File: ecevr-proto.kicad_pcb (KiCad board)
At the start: 4 copper layers, 100 x 92 mm, 218 parts, among them J1 Micro_SD_Card_Det, J1101 USB_microB, J1102 USB_C_Receptacle_USB2.0, J19 SFP, J2 Pwr_fallback, J20 SFP_CAGE, J2001 BNC, J2051 BNC, J2201 BEL_0845_2G1T_H5, J4 JTAG, J5 0821-1X1T-43-F, SW1 SW_Push, SW2101 SW_DIP_x08, U1 TXS0108EPW, U1101 USB3740B-AI9, U1102 UTC2000, U1103 FT231XS, U1104 74LVC1G00, U1105 SC185, U2001 74LVC2T45DC, U2051 74LVC2T45DC, U2101 74LVC1G06, U2102 74LVC1G06, U2103 PCA9306, U2104 24AA0x, U2201 74LVC1G06, U2202 74LVC1G06, U2301 lan9254, U6 PCA9546AD, U8 74AC125, U9 TPS2051B, X2301 FNETHE025

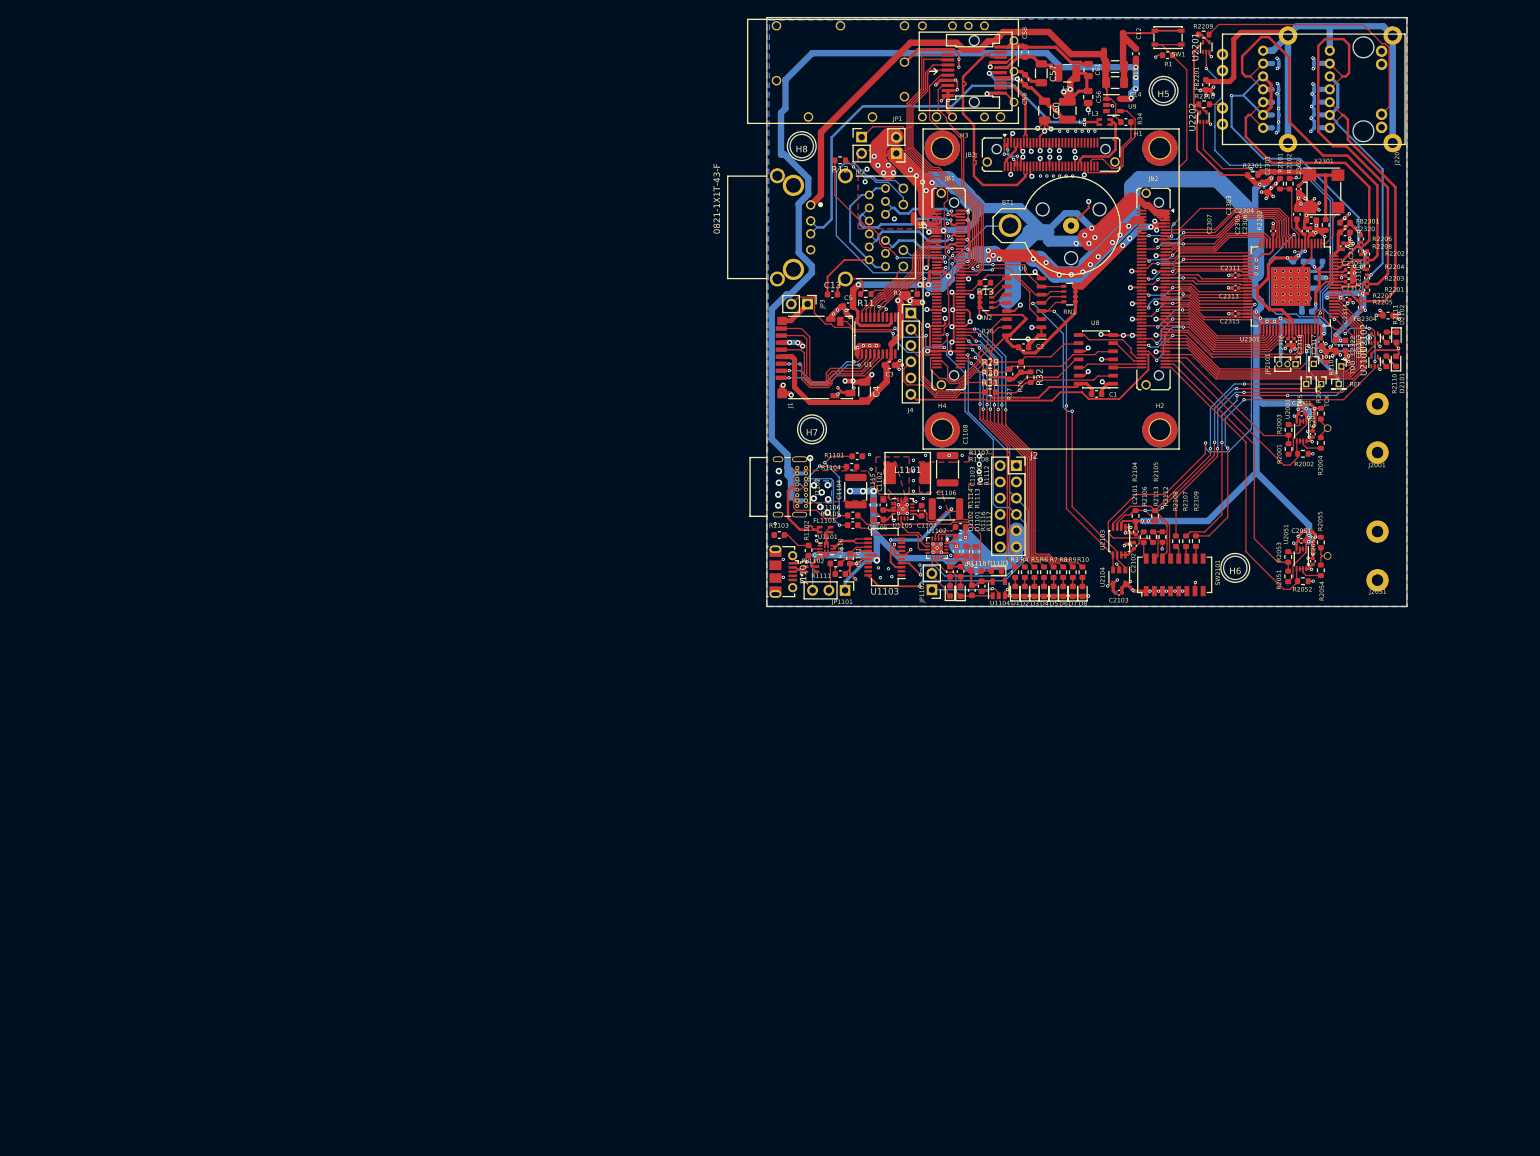
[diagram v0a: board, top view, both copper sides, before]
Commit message: WIP: (save)
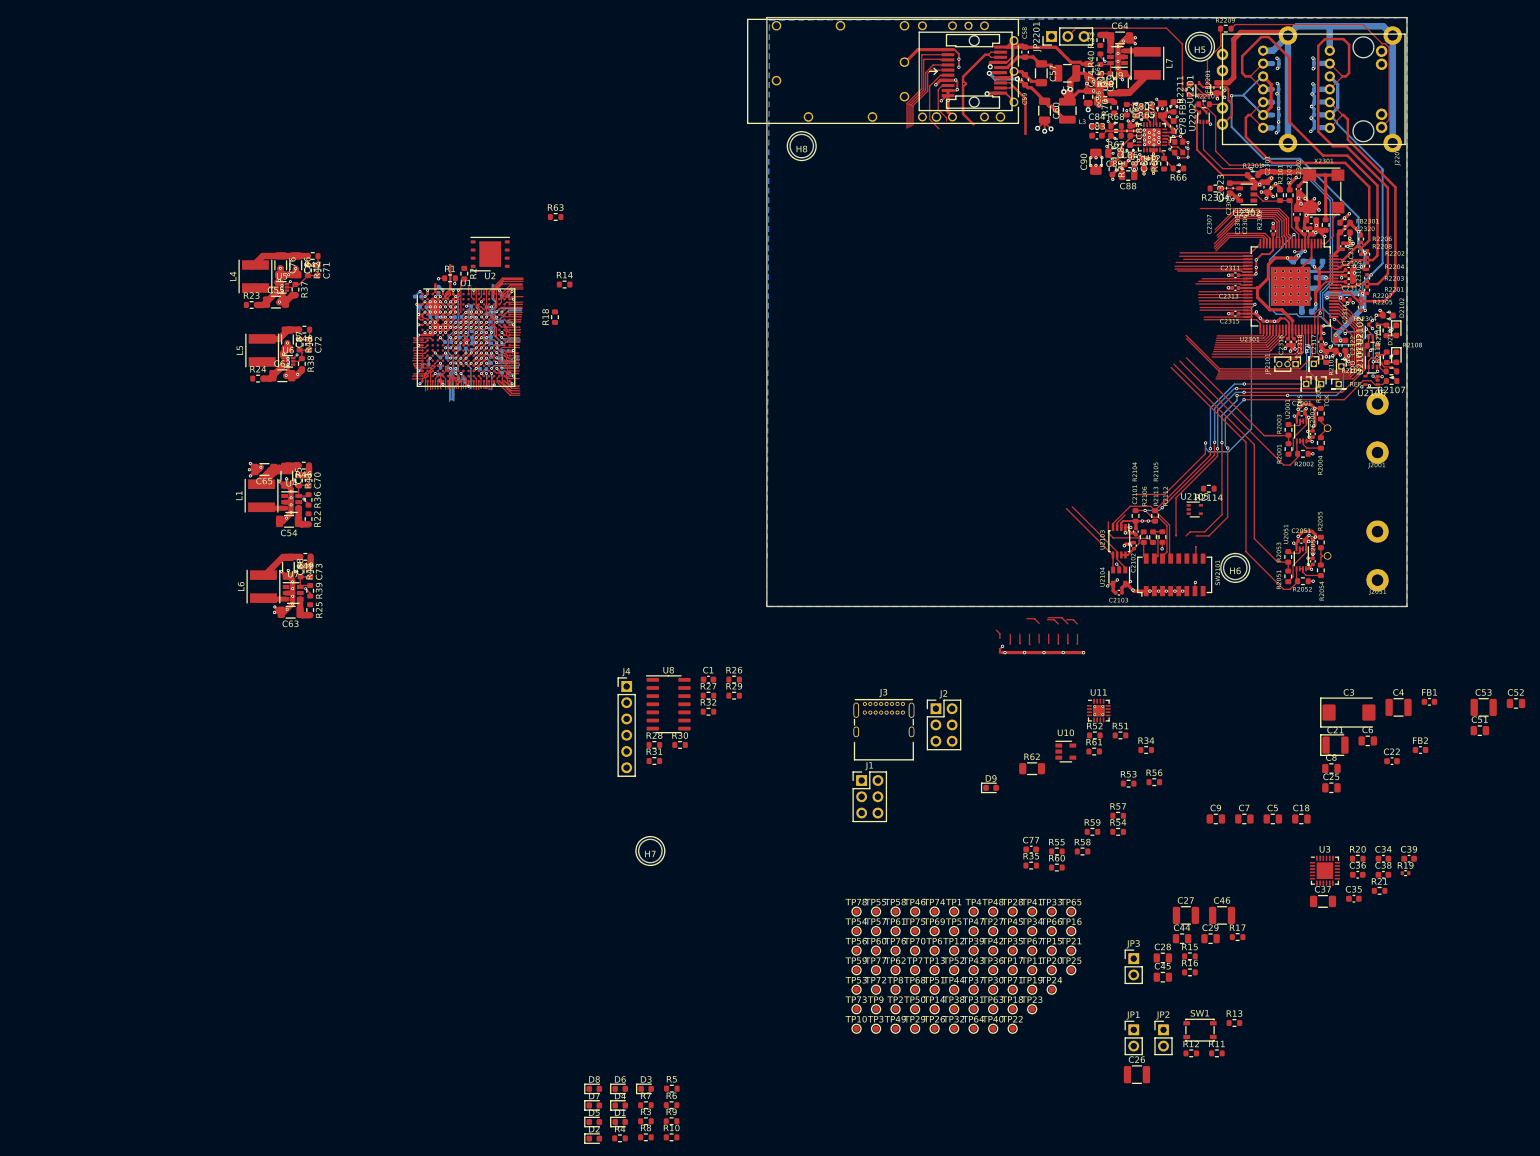
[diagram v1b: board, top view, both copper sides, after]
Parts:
- removed BT1: CR1220, Battery:BatteryHolder_Keystone_500
- removed C1101, C1102, C1103, C1105, C1107: 100nF_603, Capacitor_SMD:C_0603_1608Metric
- removed C1104, C1106, C1108: 22uF_lo_ESR, Capacitor_SMD:C_1812_4532Metric
- removed D1101, D1102, D1103: LED, LED_SMD:LED_0603_1608Metric
- removed FL1101, FL1102, FL3: EMI_Filter_LL_14, proj_footprints:WE_CNSW
- removed H1, H2, H3, H4: MountingHole_Pad, MountingHole:MountingHole_3.2mm_M3_ISO14580_Pad_TopBottom
- removed J1101: USB_microB, Connector_USB:USB_Micro-B_Molex-105017-0001
- removed J1102: USB_C_Receptacle_USB2.0, proj_footprints:USB_C_Receptacle_GCT_USB4085_smaller_holes
- removed J5: 0821-1X1T-43-F, proj_footprints:BEL_0821-1X1T-43-F
- removed JB1: LSHM-150-04_JB1, Connector_Samtec:Samtec_LSHM-150-xx.x-x-DV-S_2x50-1SH_P0.50mm_Vertical
- removed JB2: LSHM-150-04_JB2, Connector_Samtec:Samtec_LSHM-150-xx.x-x-DV-S_2x50-1SH_P0.50mm_Vertical
- removed JB3: LSHM-130-04_JB3, Connector_Samtec:Samtec_LSHM-130-xx.x-x-DV-S_2x30-1SH_P0.50mm_Vertical
- removed JP1101: Jumper_3_Bridged12, Connector_PinHeader_2.54mm:PinHeader_1x03_P2.54mm_Vertical
- removed JP1102: Jumper_NO_Small, Connector_PinHeader_2.54mm:PinHeader_1x02_P2.54mm_Vertical
- removed L1101: 1uH, proj_footprints:L_TDK_SPM6530
- removed R1101, R1104, R1109, R1110: 5k1, Resistor_SMD:R_0603_1608Metric
- removed R1102, R1103, R1116, R1117: 100k, Resistor_SMD:R_0603_1608Metric
- removed R1105, R1106, R1107, R1108, R1111: 10k, Resistor_SMD:R_0603_1608Metric
- removed R1112: 35k7, Resistor_SMD:R_0603_1608Metric
- removed R1113, R1114, R1118: 1k, Resistor_SMD:R_0603_1608Metric
- removed R1115: 1, Resistor_SMD:R_0603_1608Metric
- removed RN1, RN2: 4x4k7, Resistor_SMD:R_Array_Convex_4x0603
- removed U1101: USB3740B-AI9, Package_DFN_QFN:UQFN-10_1.6x2.1mm_P0.5mm
- removed U1102: UTC2000, proj_footprints:QFN-16-1EP_3x3mm_P0.5mm_EP1.8x1.8mm
- removed U1103: FT231XS, Package_SO:SSOP-20_3.9x8.7mm_P0.635mm
- removed U1104: 74LVC1G00, Package_TO_SOT_SMD:SOT-23-5
- removed U1105: SC185, proj_footprints:QFN-16-1EP_3x3mm_P0.5mm_EP1.8x1.8mm
- added C10: 470n, Capacitor_SMD:C_0402_1005Metric, B.Cu at (56.9, 78.0)
- added C11: 100n, Capacitor_SMD:C_0402_1005Metric, B.Cu at (48.7, 72.5)
- added C16: 470n, Capacitor_SMD:C_0402_1005Metric, B.Cu at (56.9, 83.5)
- added C17: 470n, Capacitor_SMD:C_0402_1005Metric, B.Cu at (52.5, 81.7)
- added C18: 4u7, Capacitor_SMD:C_0805_2012Metric, F.Cu at (183.5, 155.2)
- added C19: 470n, Capacitor_SMD:C_0402_1005Metric, B.Cu at (53.9, 79.5)
- added C20: 470n, Capacitor_SMD:C_0402_1005Metric, B.Cu at (53.9, 81.4)
- added C21: 100u, proj_footprints:C_pol_1210_3225Metric, F.Cu at (188.8, 143.7)
- added C22: 470n, Capacitor_SMD:C_0603_1608Metric, F.Cu at (197.7, 146.2)
- added C23: 100n, Capacitor_SMD:C_0402_1005Metric, B.Cu at (45.5, 73.6)
- added C2323: 100n, Capacitor_SMD:C_0603_1608Metric, F.Cu at (172.3, 56.6)
- added C24: 100n, Capacitor_SMD:C_0402_1005Metric, B.Cu at (46.3, 75.2)
- added C25: 4u7, Capacitor_SMD:C_0805_2012Metric, F.Cu at (188.2, 150.3)
- added C26: 47u, Capacitor_SMD:C_1210_3225Metric, F.Cu at (157.8, 195.1)
- added C27: 47u, Capacitor_SMD:C_1210_3225Metric, F.Cu at (165.5, 170.3)
- added C28: 4u7, Capacitor_SMD:C_0805_2012Metric, F.Cu at (161.9, 176.9)
- added C29: 4u7, Capacitor_SMD:C_0805_2012Metric, F.Cu at (169.3, 173.9)
- added C30: 470n, Capacitor_SMD:C_0402_1005Metric, B.Cu at (59.1, 82.1)
- added C31: 470n, Capacitor_SMD:C_0402_1005Metric, B.Cu at (59.1, 85.5)
- added C32: 470n, Capacitor_SMD:C_0402_1005Metric, B.Cu at (52.3, 86.4)
- added C33: 470n, Capacitor_SMD:C_0402_1005Metric, B.Cu at (55.7, 84.9)
- added C34: 47p, Capacitor_SMD:C_0603_1608Metric, F.Cu at (196.3, 161.4)
- added C35: 47p, Capacitor_SMD:C_0603_1608Metric, F.Cu at (191.7, 167.7)
- added C36: 100n, Capacitor_SMD:C_0603_1608Metric, F.Cu at (192.3, 163.9)
- added C37: 10u, Capacitor_SMD:C_1206_3216Metric, F.Cu at (186.9, 168.1)
- added C38: 100n, Capacitor_SMD:C_0603_1608Metric, F.Cu at (196.3, 163.9)
- added C39: 100n, Capacitor_SMD:C_0603_1608Metric, F.Cu at (200.3, 161.4)
- added C40: 470n, Capacitor_SMD:C_0402_1005Metric, B.Cu at (56.2, 75.7)
- added C41: 470n, Capacitor_SMD:C_0402_1005Metric, B.Cu at (59.1, 77.5)
- added C42: 470n, Capacitor_SMD:C_0402_1005Metric, B.Cu at (59.1, 73.5)
- added C43: 470n, Capacitor_SMD:C_0402_1005Metric, B.Cu at (54.3, 75.1)
- added C44: 4u7, Capacitor_SMD:C_0805_2012Metric, F.Cu at (164.9, 173.9)
- added C45: 4u7, Capacitor_SMD:C_0805_2012Metric, F.Cu at (161.9, 179.9)
- added C46: 47u, Capacitor_SMD:C_1210_3225Metric, F.Cu at (171.1, 170.3)
- added C47: 470n, Capacitor_SMD:C_0402_1005Metric, B.Cu at (49.5, 83.1)
- added C48: 470n, Capacitor_SMD:C_0402_1005Metric, B.Cu at (49.5, 84.7)
- added C49: 470n, Capacitor_SMD:C_0402_1005Metric, B.Cu at (46.7, 84.2)
- added C50: 470n, Capacitor_SMD:C_0402_1005Metric, B.Cu at (48.9, 86.2)
- added C51: 4u7, Capacitor_SMD:C_0805_2012Metric, F.Cu at (211.4, 141.4)
- added C52: 4u7, Capacitor_SMD:C_0805_2012Metric, F.Cu at (217.0, 137.2)
- added C53: 47u, Capacitor_SMD:C_1210_3225Metric, F.Cu at (212.0, 137.8)
- added C54: 10u, Capacitor_SMD:C_1206_3216Metric, F.Cu at (25.4, 108.7)
- added C55: 10u, Capacitor_SMD:C_1206_3216Metric, F.Cu at (23.3, 74.5)
- added C6: 4u7, Capacitor_SMD:C_0805_2012Metric, F.Cu at (193.9, 143.0)
- added C62: 10u, Capacitor_SMD:C_1206_3216Metric, F.Cu at (24.3, 86.0)
- added C63: 10u, Capacitor_SMD:C_1206_3216Metric, F.Cu at (25.6, 122.9)
- added C64: 10u, Capacitor_SMD:C_1206_3216Metric, F.Cu at (155.2, 33.2)
- added C65: 22u, Capacitor_SMD:C_1206_3216Metric, F.Cu at (21.5, 100.6)
- added C66: 22u, Capacitor_SMD:C_1206_3216Metric, F.Cu at (26.4, 68.7)
- added C67: 22u, Capacitor_SMD:C_1206_3216Metric, F.Cu at (25.1, 80.3)
- added C68: 10u, Capacitor_SMD:C_1206_3216Metric, F.Cu at (25.2, 115.8)
- added C69: 10u, Capacitor_SMD:C_1206_3216Metric, F.Cu at (155.6, 40.2)
- added C7: 4u7, Capacitor_SMD:C_0805_2012Metric, F.Cu at (174.6, 155.2)
- added C70: 86p, Capacitor_SMD:C_0603_1608Metric, F.Cu at (28.4, 102.3)
- added C71: 86p, Capacitor_SMD:C_0603_1608Metric, F.Cu at (29.8, 69.5)
- added C72: 56p, Capacitor_SMD:C_0603_1608Metric, F.Cu at (28.5, 81.1)
- added C73: 56p, Capacitor_SMD:C_0603_1608Metric, F.Cu at (28.6, 116.6)
- added C74: 130p, Capacitor_SMD:C_0603_1608Metric, F.Cu at (152.2, 39.5)
- added C75: 22u, Capacitor_SMD:C_1206_3216Metric, F.Cu at (25.0, 101.6)
- added C76: 22u, Capacitor_SMD:C_1206_3216Metric, F.Cu at (24.1, 68.7)
- added C77: 100n, Capacitor_SMD:C_0603_1608Metric, F.Cu at (141.3, 160.0)
- added C78: 100n, Capacitor_SMD:C_0603_1608Metric, F.Cu at (163.6, 47.0)
- added C79: 1u, Capacitor_SMD:C_0805_2012Metric, F.Cu at (161.8, 44.4)
- added C8: 4u7, Capacitor_SMD:C_0805_2012Metric, F.Cu at (188.2, 147.3)
- added C80: 100n, Capacitor_SMD:C_0603_1608Metric, F.Cu at (158.4, 45.4)
- added C81: 100n, Capacitor_SMD:C_0603_1608Metric, F.Cu at (156.8, 50.7)
- added C82: 100n, Capacitor_SMD:C_0603_1608Metric, F.Cu at (160.4, 52.8)
- added C83: C_Small, Capacitor_SMD:C_0603_1608Metric, F.Cu at (151.6, 48.5)
- added C84: C_Small, Capacitor_SMD:C_0603_1608Metric, F.Cu at (151.6, 47.0)
- added C85: 100n, Capacitor_SMD:C_0603_1608Metric, F.Cu at (158.9, 52.8)
- added C86: 100n, Capacitor_SMD:C_0603_1608Metric, F.Cu at (156.7, 52.9)
- added C87: 100n, Capacitor_SMD:C_0603_1608Metric, F.Cu at (156.8, 47.7)
- added C88: 1u, Capacitor_SMD:C_0805_2012Metric, F.Cu at (156.4, 54.7)
- added C89: 1u, Capacitor_SMD:C_0805_2012Metric, F.Cu at (154.3, 51.2)
- added C9: 4u7, Capacitor_SMD:C_0805_2012Metric, F.Cu at (170.1, 155.2)
- added C90: 10u, Capacitor_SMD:C_1206_3216Metric, F.Cu at (151.4, 52.5)
- added D9: LED, LED_SMD:LED_0603_1608Metric, F.Cu at (135.0, 150.3)
- added FB1: FB_250, Inductor_SMD:L_0603_1608Metric, F.Cu at (203.5, 136.9)
- added FB2: FB_250, Inductor_SMD:L_0603_1608Metric, F.Cu at (202.1, 144.4)
- added FB3: Ferrite_Bead, Inductor_SMD:L_0603_1608Metric, F.Cu at (163.6, 44.0)
- added J3: USB_C_Receptacle_USB2.0, proj_footprints:USB_C_Receptacle_GCT_USB4085_smaller_holes, F.Cu at (115.3, 137.2)
- added JP2201: 100FDb, Connector_PinHeader_2.54mm:PinHeader_1x03_P2.54mm_Vertical, F.Cu at (144.5, 33.0)
- added L1: 2u2, Inductor_SMD:L_Taiyo-Yuden_NR-50xx, F.Cu at (21.1, 104.7)
- added L4: 1u, Inductor_SMD:L_Taiyo-Yuden_NR-50xx, F.Cu at (20.1, 70.5)
- added L5: 1u, Inductor_SMD:L_Taiyo-Yuden_NR-50xx, F.Cu at (21.1, 82.0)
- added L6: 2u2, Inductor_SMD:L_Taiyo-Yuden_NR-50xx, F.Cu at (21.4, 118.9)
- added L7: 2u2, Inductor_SMD:L_Taiyo-Yuden_NR-50xx, F.Cu at (159.4, 37.1)
- added R14: 1k, Resistor_SMD:R_0603_1608Metric, F.Cu at (68.4, 71.7)
- added R15: 2k4, Resistor_SMD:R_0603_1608Metric, F.Cu at (166.1, 176.7)
- added R16: 2k4, Resistor_SMD:R_0603_1608Metric, F.Cu at (166.1, 179.2)
- added R17: 2k4, Resistor_SMD:R_0603_1608Metric, F.Cu at (173.5, 173.7)
- added R18: 50, Resistor_SMD:R_0603_1608Metric, F.Cu at (66.9, 76.8)
- added R19: 0, Resistor_SMD:R_0402_1005Metric, F.Cu at (199.8, 163.7)
- added R20: 27, Resistor_SMD:R_0603_1608Metric, F.Cu at (192.3, 161.4)
- added R21: 27, Resistor_SMD:R_0603_1608Metric, F.Cu at (195.7, 166.4)
- added R2114: 100k, Resistor_SMD:R_0603_1608Metric, F.Cu at (169.1, 103.6)
- added R22: 10k, Resistor_SMD:R_0603_1608Metric, F.Cu at (28.4, 108.3)
- added R2211: 100, Resistor_SMD:R_0603_1608Metric, F.Cu at (166.0, 41.2)
- added R23: 10k, Resistor_SMD:R_0603_1608Metric, F.Cu at (19.5, 74.9)
- added R2304: 50, Resistor_SMD:R_0603_1608Metric, F.Cu at (170.1, 56.7)
- added R24: 10k, Resistor_SMD:R_0603_1608Metric, F.Cu at (20.5, 86.4)
- added R25: 10k, Resistor_SMD:R_0603_1608Metric, F.Cu at (28.6, 122.5)
- added R33: 10k, Resistor_SMD:R_0603_1608Metric, F.Cu at (152.1, 33.5)
- added R35: 10k, Resistor_SMD:R_0603_1608Metric, F.Cu at (141.3, 162.5)
- added R36: 24k, Resistor_SMD:R_0603_1608Metric, F.Cu at (28.4, 105.3)
- added R37: 24k, Resistor_SMD:R_0603_1608Metric, F.Cu at (26.4, 72.5)
- added R38: 24k, Resistor_SMD:R_0603_1608Metric, F.Cu at (27.4, 84.1)
- added R39: 12k, Resistor_SMD:R_0603_1608Metric, F.Cu at (28.6, 119.5)
- added R40: 45.9k, Resistor_SMD:R_0603_1608Metric, F.Cu at (152.1, 36.5)
- added R41: 16k, Resistor_SMD:R_0603_1608Metric, F.Cu at (26.9, 102.3)
- added R42: 16k, Resistor_SMD:R_0603_1608Metric, F.Cu at (28.3, 69.5)
- added R43: 24k, Resistor_SMD:R_0603_1608Metric, F.Cu at (27.0, 81.1)
- added R44: 24k, Resistor_SMD:R_0603_1608Metric, F.Cu at (27.1, 116.5)
- added R45: 10.2k, Resistor_SMD:R_0603_1608Metric, F.Cu at (153.7, 39.5)
- added R46: 0, Resistor_SMD:R_0603_1608Metric, F.Cu at (27.6, 100.0)
- added R47: 0, Resistor_SMD:R_0603_1608Metric, F.Cu at (29.1, 67.2)
- added R48: 0, Resistor_SMD:R_0603_1608Metric, F.Cu at (27.8, 78.8)
- added R49: 0, Resistor_SMD:R_0603_1608Metric, F.Cu at (27.9, 114.2)
- added R50: 0, Resistor_SMD:R_0603_1608Metric, F.Cu at (152.9, 41.8)
- added R51: 1k, Resistor_SMD:R_0603_1608Metric, F.Cu at (155.2, 142.2)
- added R52: 100k, Resistor_SMD:R_0603_1608Metric, F.Cu at (151.2, 142.2)
- added R53: 100k, Resistor_SMD:R_0603_1608Metric, F.Cu at (156.5, 149.7)
- added R54: 10k, Resistor_SMD:R_0603_1608Metric, F.Cu at (154.9, 157.2)
- added R55: 10k, Resistor_SMD:R_0603_1608Metric, F.Cu at (145.3, 160.3)
- added R56: 5k1, Resistor_SMD:R_0603_1608Metric, F.Cu at (160.5, 149.4)
- added R57: 5k1, Resistor_SMD:R_0603_1608Metric, F.Cu at (154.9, 154.7)
- added R58: 10k, Resistor_SMD:R_0603_1608Metric, F.Cu at (149.3, 160.3)
- added R59: 10k, Resistor_SMD:R_0603_1608Metric, F.Cu at (150.9, 157.2)
- added R60: 5k1, Resistor_SMD:R_0603_1608Metric, F.Cu at (145.3, 162.8)
- added R61: 35k7, Resistor_SMD:R_0603_1608Metric, F.Cu at (151.1, 144.7)
- added R62: 0.01, Resistor_SMD:R_1206_3216Metric, F.Cu at (141.4, 147.3)
- added R63: 4k7, Resistor_SMD:R_0603_1608Metric, F.Cu at (67.0, 61.1)
- added R64: 10k, Resistor_SMD:R_0603_1608Metric, F.Cu at (156.2, 44.4)
- added R65: 10k, Resistor_SMD:R_0603_1608Metric, F.Cu at (159.3, 43.8)
- added R66: 1k78, Resistor_SMD:R_0603_1608Metric, F.Cu at (164.3, 53.6)
- added R67: 50, Resistor_SMD:R_0603_1608Metric, F.Cu at (154.6, 48.5)
- added R68: 50, Resistor_SMD:R_0603_1608Metric, F.Cu at (154.6, 47.0)
- added R69: 33, Resistor_SMD:R_0603_1608Metric, F.Cu at (162.1, 52.8)
- added R70: 0, Resistor_SMD:R_0603_1608Metric, F.Cu at (154.3, 44.1)
- added R71: 0, Resistor_SMD:R_0603_1608Metric, F.Cu at (154.0, 53.7)
- added TP1: TestPoint_Small, TestPoint:TestPoint_Pad_D1.0mm, F.Cu at (129.3, 169.7)
- added TP10: TestPoint_Small, TestPoint:TestPoint_Pad_D1.0mm, F.Cu at (114.0, 188.0)
- added TP11: TestPoint_Small, TestPoint:TestPoint_Pad_D1.0mm, F.Cu at (141.5, 178.8)
- added TP12: TestPoint_Small, TestPoint:TestPoint_Pad_D1.0mm, F.Cu at (129.3, 175.8)
- added TP13: TestPoint_Small, TestPoint:TestPoint_Pad_D1.0mm, F.Cu at (126.2, 178.8)
- added TP14: TestPoint_Small, TestPoint:TestPoint_Pad_D1.0mm, F.Cu at (126.2, 184.9)
- added TP15: TestPoint_Small, TestPoint:TestPoint_Pad_D1.0mm, F.Cu at (144.5, 175.8)
- added TP16: TestPoint_Small, TestPoint:TestPoint_Pad_D1.0mm, F.Cu at (147.6, 172.7)
- added TP17: TestPoint_Small, TestPoint:TestPoint_Pad_D1.0mm, F.Cu at (138.4, 178.8)
- added TP18: TestPoint_Small, TestPoint:TestPoint_Pad_D1.0mm, F.Cu at (138.4, 184.9)
- added TP19: TestPoint_Small, TestPoint:TestPoint_Pad_D1.0mm, F.Cu at (141.5, 181.9)
- added TP2: TestPoint_Small, TestPoint:TestPoint_Pad_D1.0mm, F.Cu at (120.1, 184.9)
- added TP20: TestPoint_Small, TestPoint:TestPoint_Pad_D1.0mm, F.Cu at (144.5, 178.8)
- added TP21: TestPoint_Small, TestPoint:TestPoint_Pad_D1.0mm, F.Cu at (147.6, 175.8)
- added TP22: TestPoint_Small, TestPoint:TestPoint_Pad_D1.0mm, F.Cu at (138.4, 188.0)
- added TP23: TestPoint_Small, TestPoint:TestPoint_Pad_D1.0mm, F.Cu at (141.5, 184.9)
- added TP24: TestPoint_Small, TestPoint:TestPoint_Pad_D1.0mm, F.Cu at (144.5, 181.9)
- added TP25: TestPoint_Small, TestPoint:TestPoint_Pad_D1.0mm, F.Cu at (147.6, 178.8)
- added TP26: TestPoint_Small, TestPoint:TestPoint_Pad_D1.0mm, F.Cu at (126.2, 188.0)
- added TP27: TestPoint_Small, TestPoint:TestPoint_Pad_D1.0mm, F.Cu at (135.4, 172.7)
- added TP28: TestPoint_Small, TestPoint:TestPoint_Pad_D1.0mm, F.Cu at (138.4, 169.7)
- added TP29: TestPoint_Small, TestPoint:TestPoint_Pad_D1.0mm, F.Cu at (123.2, 188.0)
- added TP3: TestPoint_Small, TestPoint:TestPoint_Pad_D1.0mm, F.Cu at (117.1, 188.0)
- added TP30: TestPoint_Small, TestPoint:TestPoint_Pad_D1.0mm, F.Cu at (135.4, 181.9)
- added TP31: TestPoint_Small, TestPoint:TestPoint_Pad_D1.0mm, F.Cu at (132.3, 184.9)
- added TP32: TestPoint_Small, TestPoint:TestPoint_Pad_D1.0mm, F.Cu at (129.3, 188.0)
- added TP33: TestPoint_Small, TestPoint:TestPoint_Pad_D1.0mm, F.Cu at (144.5, 169.7)
- added TP34: TestPoint_Small, TestPoint:TestPoint_Pad_D1.0mm, F.Cu at (141.5, 172.7)
- added TP35: TestPoint_Small, TestPoint:TestPoint_Pad_D1.0mm, F.Cu at (138.4, 175.8)
- added TP36: TestPoint_Small, TestPoint:TestPoint_Pad_D1.0mm, F.Cu at (135.4, 178.8)
- added TP37: TestPoint_Small, TestPoint:TestPoint_Pad_D1.0mm, F.Cu at (132.3, 181.9)
- added TP38: TestPoint_Small, TestPoint:TestPoint_Pad_D1.0mm, F.Cu at (129.3, 184.9)
- added TP39: TestPoint_Small, TestPoint:TestPoint_Pad_D1.0mm, F.Cu at (132.3, 175.8)
- added TP4: TestPoint_Small, TestPoint:TestPoint_Pad_D1.0mm, F.Cu at (132.3, 169.7)
- added TP40: TestPoint_Small, TestPoint:TestPoint_Pad_D1.0mm, F.Cu at (135.4, 188.0)
- added TP41: TestPoint_Small, TestPoint:TestPoint_Pad_D1.0mm, F.Cu at (141.5, 169.7)
- added TP42: TestPoint_Small, TestPoint:TestPoint_Pad_D1.0mm, F.Cu at (135.4, 175.8)
- added TP43: TestPoint_Small, TestPoint:TestPoint_Pad_D1.0mm, F.Cu at (132.3, 178.8)
- added TP44: TestPoint_Small, TestPoint:TestPoint_Pad_D1.0mm, F.Cu at (129.3, 181.9)
- added TP45: TestPoint_Small, TestPoint:TestPoint_Pad_D1.0mm, F.Cu at (138.4, 172.7)
- added TP46: TestPoint_Small, TestPoint:TestPoint_Pad_D1.0mm, F.Cu at (123.2, 169.7)
- added TP47: TestPoint_Small, TestPoint:TestPoint_Pad_D1.0mm, F.Cu at (132.3, 172.7)
- added TP48: TestPoint_Small, TestPoint:TestPoint_Pad_D1.0mm, F.Cu at (135.4, 169.7)
- added TP49: TestPoint_Small, TestPoint:TestPoint_Pad_D1.0mm, F.Cu at (120.1, 188.0)
- added TP5: TestPoint_Small, TestPoint:TestPoint_Pad_D1.0mm, F.Cu at (129.3, 172.7)
- added TP50: TestPoint_Small, TestPoint:TestPoint_Pad_D1.0mm, F.Cu at (123.2, 184.9)
- added TP51: TestPoint_Small, TestPoint:TestPoint_Pad_D1.0mm, F.Cu at (126.2, 181.9)
- added TP52: TestPoint_Small, TestPoint:TestPoint_Pad_D1.0mm, F.Cu at (129.3, 178.8)
- added TP53: TestPoint_Small, TestPoint:TestPoint_Pad_D1.0mm, F.Cu at (114.0, 181.9)
- added TP54: TestPoint_Small, TestPoint:TestPoint_Pad_D1.0mm, F.Cu at (114.0, 172.7)
- added TP55: TestPoint_Small, TestPoint:TestPoint_Pad_D1.0mm, F.Cu at (117.1, 169.7)
- added TP56: TestPoint_Small, TestPoint:TestPoint_Pad_D1.0mm, F.Cu at (114.0, 175.8)
- added TP57: TestPoint_Small, TestPoint:TestPoint_Pad_D1.0mm, F.Cu at (117.1, 172.7)
- added TP58: TestPoint_Small, TestPoint:TestPoint_Pad_D1.0mm, F.Cu at (120.1, 169.7)
- added TP59: TestPoint_Small, TestPoint:TestPoint_Pad_D1.0mm, F.Cu at (114.0, 178.8)
- added TP6: TestPoint_Small, TestPoint:TestPoint_Pad_D1.0mm, F.Cu at (126.2, 175.8)
- added TP60: TestPoint_Small, TestPoint:TestPoint_Pad_D1.0mm, F.Cu at (117.1, 175.8)
- added TP61: TestPoint_Small, TestPoint:TestPoint_Pad_D1.0mm, F.Cu at (120.1, 172.7)
- added TP62: TestPoint_Small, TestPoint:TestPoint_Pad_D1.0mm, F.Cu at (120.1, 178.8)
- added TP63: TestPoint_Small, TestPoint:TestPoint_Pad_D1.0mm, F.Cu at (135.4, 184.9)
- added TP64: TestPoint_Small, TestPoint:TestPoint_Pad_D1.0mm, F.Cu at (132.3, 188.0)
- added TP65: TestPoint_Small, TestPoint:TestPoint_Pad_D1.0mm, F.Cu at (147.6, 169.7)
- added TP66: TestPoint_Small, TestPoint:TestPoint_Pad_D1.0mm, F.Cu at (144.5, 172.7)
- added TP67: TestPoint_Small, TestPoint:TestPoint_Pad_D1.0mm, F.Cu at (141.5, 175.8)
- added TP68: TestPoint_Small, TestPoint:TestPoint_Pad_D1.0mm, F.Cu at (123.2, 181.9)
- added TP69: TestPoint_Small, TestPoint:TestPoint_Pad_D1.0mm, F.Cu at (126.2, 172.7)
- added TP7: TestPoint_Small, TestPoint:TestPoint_Pad_D1.0mm, F.Cu at (123.2, 178.8)
- added TP70: TestPoint_Small, TestPoint:TestPoint_Pad_D1.0mm, F.Cu at (123.2, 175.8)
- added TP71: TestPoint_Small, TestPoint:TestPoint_Pad_D1.0mm, F.Cu at (138.4, 181.9)
- added TP72: TestPoint_Small, TestPoint:TestPoint_Pad_D1.0mm, F.Cu at (117.1, 181.9)
- added TP73: TestPoint_Small, TestPoint:TestPoint_Pad_D1.0mm, F.Cu at (114.0, 184.9)
- added TP74: TestPoint_Small, TestPoint:TestPoint_Pad_D1.0mm, F.Cu at (126.2, 169.7)
- added TP75: TestPoint_Small, TestPoint:TestPoint_Pad_D1.0mm, F.Cu at (123.2, 172.7)
- added TP76: TestPoint_Small, TestPoint:TestPoint_Pad_D1.0mm, F.Cu at (120.1, 175.8)
- added TP77: TestPoint_Small, TestPoint:TestPoint_Pad_D1.0mm, F.Cu at (117.1, 178.8)
- added TP78: TestPoint_Small, TestPoint:TestPoint_Pad_D1.0mm, F.Cu at (114.0, 169.7)
- added TP8: TestPoint_Small, TestPoint:TestPoint_Pad_D1.0mm, F.Cu at (120.1, 181.9)
- added TP9: TestPoint_Small, TestPoint:TestPoint_Pad_D1.0mm, F.Cu at (117.1, 184.9)
- added U10: 74LVC1G02, Package_TO_SOT_SMD:SOT-23-5, F.Cu at (146.7, 144.7)
- added U11: UTC2000, Package_DFN_QFN:QFN-16-1EP_3x3mm_P0.5mm_EP1.75x1.75mm_ThermalVias, F.Cu at (151.9, 138.3)
- added U12: 5P49V6965, Package_DFN_QFN:QFN-24-1EP_4x4mm_P0.5mm_EP2.8x2.8mm, F.Cu at (160.2, 48.7)
- added U2: AT25SL641, Package_SON:WSON-8-1EP_6x5mm_P1.27mm_EP3.4x4mm, F.Cu at (56.8, 67.0)
- added U2105: 74AHC1T86, Package_TO_SOT_SMD:SOT-353_SC-70-5, F.Cu at (166.8, 106.8)
- added U2106: 74AHC1T86, Package_TO_SOT_SMD:SOT-353_SC-70-5, F.Cu at (194.5, 86.7)
- added U2302: SN74LV1T34DBV, Package_TO_SOT_SMD:SOT-23-5, F.Cu at (175.0, 57.6)
- added U3: FT240XQ, Package_DFN_QFN:QFN-24-1EP_4x4mm_P0.5mm_EP2.6x2.6mm, F.Cu at (187.2, 163.3)
- added U4: TLV62569ADDC, Package_TO_SOT_SMD:SOT-23-6, F.Cu at (25.8, 105.7)
- added U5: TPS62A01A-SOT563, Package_TO_SOT_SMD:SOT-563, F.Cu at (24.2, 72.2)
- added U7: TLV62569ADDC, Package_TO_SOT_SMD:SOT-23-6, F.Cu at (26.0, 119.9)
- added Y1: 25MHz, Crystal:Crystal_SMD_Abracon_ABM10-4Pin_2.5x2.0mm, F.Cu at (164.3, 50.2)
- C12, C13, C2: value 100nF_603 -> 470n; footprint Capacitor_SMD:C_0603_1608Metric -> Capacitor_SMD:C_0402_1005Metric; moved to B.Cu
- C14: value 47uF, 10V -> 470n; footprint Capacitor_SMD:C_1206_3216Metric -> Capacitor_SMD:C_0402_1005Metric; moved to B.Cu
- C15: value 47uF, 10V -> 100n; footprint Capacitor_SMD:C_1206_3216Metric -> Capacitor_SMD:C_0402_1005Metric; moved to B.Cu
- C3: value 100nF_603 -> 330u; footprint Capacitor_SMD:C_0603_1608Metric -> Capacitor_Tantalum_SMD:CP_EIA-7343-30_AVX-N
- C4: value 10u -> 47u; footprint Capacitor_SMD:C_1206_3216Metric -> Capacitor_SMD:C_1210_3225Metric
- C5: value 100nF_603 -> 4u7; footprint Capacitor_SMD:C_0603_1608Metric -> Capacitor_SMD:C_0805_2012Metric
- J1: value Micro_SD_Card_Det -> PEN_SEL; footprint proj_footprints:microSD_HC_Hirose_DM3D-SF_smaller_crtyd -> Connector_PinHeader_2.54mm:PinHeader_2x03_P2.54mm_Vertical
- J2: value Pwr_fallback -> PEN_SEL; footprint Connector_PinSocket_2.54mm:PinSocket_2x06_P2.54mm_Vertical -> Connector_PinHeader_2.54mm:PinHeader_2x03_P2.54mm_Vertical
- JP1: value TEST -> JTAG_boot
- JP2: value Jumper -> INITb
- JP3: value Jumper_NO_Small -> PUDC_dis
- R1: value 10k -> 100
- R11: value 100 -> 1k
- R12: value 100 -> 4k7
- R13: value 10k -> 4k7
- R2: value 10k -> 50
- R2107: value 1k -> 100k
- R34: value 10k -> 0
- SW1: value SW_Push -> PROG
- U1: value TXS0108EPW -> XC7A35T-CSG325; footprint Package_SO:TSSOP-20_4.4x6.5mm_P0.65mm -> Package_BGA:Xilinx_CSG325
- U2101, U2102, U2201: value 74LVC1G06 -> 74AHC1T86; footprint proj_footprints:SOT-5x3 -> Package_TO_SOT_SMD:SOT-353_SC-70-5
- U6: value PCA9546AD -> TPS62A01A-SOT563; footprint Package_SO:SOIC-16_3.9x9.9mm_P1.27mm -> Package_TO_SOT_SMD:SOT-563
- U8: value 74AC125 -> 74ALVC125
- U9: value TPS2051B -> TLV62569ADDC; footprint Package_TO_SOT_SMD:SOT-23-5 -> Package_TO_SOT_SMD:SOT-23-6
- moved SW1 155.1 mm to (167.7, 188.2)
- moved R12 149.9 mm to (166.3, 191.8), turned to 0 degrees
- moved JP2 147.2 mm to (162.0, 188.1)
- moved JP1 141.8 mm to (157.3, 188.1), turned to 0 degrees
- moved R11 130.7 mm to (170.3, 191.8), turned to 0 degrees
- moved R13 122.0 mm to (173.0, 187.1), turned to 0 degrees
- moved R1 117.4 mm to (50.5, 70.7)
- moved U6 115.3 mm to (25.2, 83.7), turned to 0 degrees
- moved JP3 114.3 mm to (157.3, 177.0), turned to 0 degrees
- moved C12 113.6 mm to (51.8, 76.8), turned to 0 degrees
- moved C15 113.5 mm to (47.9, 76.8), turned to 180 degrees
- moved C14 111.8 mm to (50.2, 80.7), turned to 180 degrees
- moved R8 109.8 mm to (81.1, 204.9), turned to 0 degrees
- moved D7 109.7 mm to (73.0, 200.0), turned to 0 degrees
- moved D5 109.6 mm to (73.0, 202.5), turned to 0 degrees
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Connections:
- C1 pad 1: OTG_ID -> GND
- C1 pad 2: +3V3 -> +1V8
- C12 pad 1: +5V -> +1V0
- C12 pad 2: OTG_ID -> GND
- C13 pad 1: Net-(C13-Pad1) -> +1V8
- C13 pad 2: OTG_ID -> GND
- C14 pad 1: Net-(C14-Pad1) -> +1V0
- C14 pad 2: OTG_ID -> GND
- C15 pad 1: Net-(C14-Pad1) -> /fpga/1V0_MGT
- C15 pad 2: OTG_ID -> GND
- C2 pad 1: +3V3 -> Net-(C2-Pad1)
- C2 pad 2: OTG_ID -> /fpga/fpga_bank0_cfg/AGND
- C2001 pad 2: OTG_ID -> GND
- C2002 pad 2: OTG_ID -> GND
- C2051 pad 2: OTG_ID -> GND
- C2052 pad 2: OTG_ID -> GND
- C2101 pad 2: OTG_ID -> GND
- C2102 pad 2: OTG_ID -> GND
- C2103 pad 1: +3V3 -> +1V8
- C2103 pad 2: OTG_ID -> GND
- C2201 pad 2: OTG_ID -> GND
- C2202 pad 2: OTG_ID -> GND
- C2203 pad 2: OTG_ID -> GND
- C2204 pad 2: OTG_ID -> GND
- C2205 pad 2: OTG_ID -> GND
- C2206 pad 2: OTG_ID -> GND
- C2207 pad 2: OTG_ID -> GND
- C2208 pad 2: OTG_ID -> GND
- C2209 pad 2: OTG_ID -> GND
- C2210 pad 2: OTG_ID -> GND
- C2301 pad 2: OTG_ID -> GND
- C2302 pad 2: OTG_ID -> GND
- C2303 pad 2: OTG_ID -> GND
- C2304 pad 2: OTG_ID -> GND
- C2305 pad 2: OTG_ID -> GND
- C2306 pad 2: OTG_ID -> GND
- C2307 pad 2: OTG_ID -> GND
- C2308 pad 1: OTG_ID -> GND
- C2309 pad 1: OTG_ID -> GND
- C2310 pad 1: OTG_ID -> GND
- C2311 pad 2: OTG_ID -> GND
- C2312 pad 1: OTG_ID -> GND
- C2313 pad 2: OTG_ID -> GND
- C2314 pad 1: OTG_ID -> GND
- C2315 pad 2: OTG_ID -> GND
- C2316 pad 2: OTG_ID -> GND
- C2317 pad 2: OTG_ID -> GND
- C2318 pad 2: OTG_ID -> GND
- C2319 pad 2: OTG_ID -> GND
- C2320 pad 2: OTG_ID -> GND
- C2321 pad 2: OTG_ID -> GND
- C2322 pad 2: OTG_ID -> GND
- C3 pad 1: +3V3 -> +1V0
- C3 pad 2: OTG_ID -> GND
- C4 pad 1: OTG_ID -> +1V8
- C4 pad 2: +3V3 -> GND
- C5 pad 2: OTG_ID -> GND
- C56 pad 2: OTG_ID -> GND
- C57 pad 2: OTG_ID -> GND
- C58 pad 2: OTG_ID -> GND
- C59 pad 2: OTG_ID -> GND
- C60 pad 2: OTG_ID -> GND
- C61 pad 2: OTG_ID -> GND
- D1 pad 1: OTG_ID -> GND
- D2 pad 1: OTG_ID -> GND
- D2101 pad 1: Net-(D2101-Pad1) -> GND
- D2101 pad 2: +3V3 -> Net-(D2101-Pad2)
- D2102 pad 1: Net-(D2102-Pad1) -> GND
- D2102 pad 2: +3V3 -> Net-(D2102-Pad2)
- D3 pad 1: OTG_ID -> GND
- D4 pad 1: OTG_ID -> GND
- D5 pad 1: OTG_ID -> GND
- D6 pad 1: OTG_ID -> GND
- D7 pad 1: OTG_ID -> GND
- D8 pad 1: OTG_ID -> GND
- FB2201 pad 2: OTG_ID -> GND
- J1 pad 2: Net-(J1-Pad2) -> /power/1A5
- J1 pad 3: Net-(J1-Pad3) -> Net-(J1-Pad1)
- J1 pad 4: +3V3 -> /power/3A0
- J1 pad 5: Net-(J1-Pad5) -> Net-(J1-Pad1)
- J1 pad 6: OTG_ID -> GND
- J19 pad 1: OTG_ID -> GND
- J19 pad 10: OTG_ID -> GND
- J19 pad 11: OTG_ID -> GND
- J19 pad 14: OTG_ID -> GND
- J19 pad 17: OTG_ID -> GND
- J19 pad 18: MGT_TX1_N -> MGT_TX1_P
- J19 pad 19: MGT_TX1_P -> MGT_TX1_N
- J19 pad 20: OTG_ID -> GND
- J19 pad 7: OTG_ID -> GND
- J19 pad 9: OTG_ID -> GND
- J2 pad 1: +3V3_PWR_OUT -> Net-(J2-Pad1)
- J2 pad 2: OTG_ID -> USB_BCDb
- J2 pad 3: +3V3_PWR_OUT -> Net-(J2-Pad1)
- J2 pad 4: OTG_ID -> USB_PWRENb
- J2 pad 5: UART_RX_MIO14 -> Net-(J2-Pad1)
- J2 pad 6: OTG_ID -> GND
- J20 pad 1: OTG_ID -> GND
- J20 pad 10: OTG_ID -> GND
- J20 pad 11: OTG_ID -> GND
- J20 pad 12: OTG_ID -> GND
- J20 pad 13: OTG_ID -> GND
- J20 pad 14: OTG_ID -> GND
- J20 pad 15: OTG_ID -> GND
- J20 pad 16: OTG_ID -> GND
- J20 pad 17: OTG_ID -> GND
- J20 pad 18: OTG_ID -> GND
- J20 pad 19: OTG_ID -> GND
- J20 pad 2: OTG_ID -> GND
- J20 pad 20: OTG_ID -> GND
- J20 pad 3: OTG_ID -> GND
- J20 pad 4: OTG_ID -> GND
- J20 pad 5: OTG_ID -> GND
- J20 pad 6: OTG_ID -> GND
- J20 pad 7: OTG_ID -> GND
- J20 pad 8: OTG_ID -> GND
- J20 pad 9: OTG_ID -> GND
- J2001 pad 2: OTG_ID -> GND
- J2051 pad 2: OTG_ID -> GND
- J2201 pad 15: +3V3 -> Net-(J2201-Pad15)
- J2201 pad 16: Net-(J2201-Pad16) -> GND
- J4 pad 5: OTG_ID -> GND
- J4 pad 6: VREF_JTAG -> +1V8
- JP1 pad 1: +3V3_PWR_OUT -> +1V8
- JP1 pad 2: +3V3 -> Net-(JP1-Pad2)
- JP2 pad 1: /B2B Connector/MODE -> Net-(JP2-Pad1)
- JP2 pad 2: OTG_ID -> GND
- JP2101 pad 1: OTG_ID -> GND
- JP3 pad 1: OTG_ID -> +1V8
- JP3 pad 2: MIO_0 -> Net-(JP3-Pad2)
- R1 pad 1: +3V3 -> /fpga/1V2_MGT
- R1 pad 2: /B2B Connector/RESIN -> Net-(R1-Pad2)
- R11 pad 1: Net-(J5-Pad19) -> GND
- R11 pad 2: OTG_ID -> Net-(JP1-Pad2)
- R12 pad 1: Net-(J5-Pad21) -> Net-(R12-Pad1)
- R12 pad 2: B13_L3_N -> +1V8
- R13 pad 1: +3V3 -> Net-(JP2-Pad1)
- R13 pad 2: B13_L8_N -> +1V8
- R2 pad 1: +3V3 -> /fpga/fpga_bank0_cfg/CCLK
- R2 pad 2: /B2B Connector/EN1 -> Net-(R2-Pad2)
- R2002 pad 2: OTG_ID -> GND
- R2005 pad 2: OTG_ID -> GND
- R2052 pad 2: OTG_ID -> GND
- R2055 pad 2: OTG_ID -> GND
- R2101 pad 2: OTG_ID -> GND
- R2103 pad 2: OTG_ID -> GND
- R2107 pad 1: /lan9254/LINKACT0 -> +3V3
- R2110 pad 1: Net-(D2101-Pad1) -> Net-(D2101-Pad2)
- R2111 pad 1: Net-(D2102-Pad1) -> Net-(D2102-Pad2)
- R2113 pad 1: +3V3 -> +1V8
- R2209 pad 1: Net-(J2201-Pad16) -> Net-(J2201-Pad15)
- R2303 pad 1: OTG_ID -> GND
- R26 pad 1: +3V3 -> +1V8
- R27 pad 1: +3V3 -> +1V8
- R32 pad 1: +3V3 -> +1V8
- R34 pad 1: USB_VBUS -> Net-(R33-Pad1)
- R34 pad 2: Net-(C14-Pad1) -> Net-(R34-Pad2)
- SW1 pad 1: OTG_ID -> Net-(R12-Pad1)
- SW1 pad 2: /B2B Connector/RESIN -> GND
- SW2101 pad 1: OTG_ID -> GND
- SW2101 pad 10: Net-(R2109-Pad2) -> Net-(SW2101-Pad10)
- SW2101 pad 12: Net-(R2108-Pad2) -> Net-(R2114-Pad2)
- SW2101 pad 2: OTG_ID -> GND
- SW2101 pad 3: OTG_ID -> GND
- SW2101 pad 4: OTG_ID -> GND
- SW2101 pad 5: OTG_ID -> GND
- SW2101 pad 6: OTG_ID -> GND
- SW2101 pad 7: +3V3 -> Net-(SW2101-Pad7)
- U2001 pad 4: OTG_ID -> GND
- U2051 pad 4: OTG_ID -> GND
- U2101 pad 1: Net-(U2101-Pad1) -> Net-(R2109-Pad2)
- U2101 pad 3: OTG_ID -> GND
- U2102 pad 1: Net-(U2102-Pad1) -> Net-(R2108-Pad2)
- U2102 pad 3: OTG_ID -> GND
- U2102 pad 5: +1V8 -> +3V3
- U2103 pad 1: OTG_ID -> GND
- U2104 pad 2: OTG_ID -> GND
- U2104 pad 4: +3V3 -> +1V8
- U2104 pad 5: OTG_ID -> GND
- U2201 pad 3: OTG_ID -> GND
- U2201 pad 5: +1V8 -> +3V3
- U2202 pad 3: OTG_ID -> GND
- U2301 pad 4: OTG_ID -> GND
- U2301 pad 81: OTG_ID -> GND
- U6 pad 1: OTG_ID -> GND
- U6 pad 2: OTG_ID -> Net-(L5-Pad1)
- U6 pad 3: B13_L8_N -> +5V
- U6 pad 4: SDA0 -> Net-(R24-Pad1)
- U6 pad 5: SCL0 -> Net-(C72-Pad2)
- U6 pad 6: SDA1 -> Net-(R25-Pad1)
- U8 pad 1: OTG_ID -> GND
- U8 pad 10: OTG_ID -> GND
- U8 pad 13: OTG_ID -> GND
- U8 pad 14: +3V3 -> +1V8
- U8 pad 4: OTG_ID -> GND
- U8 pad 7: OTG_ID -> GND
- U9 pad 1: Net-(C14-Pad1) -> Net-(R33-Pad1)
- U9 pad 2: OTG_ID -> GND
- U9 pad 4: VBUS_V_EN -> +5V
- U9 pad 5: +5V -> Net-(R35-Pad1)
- X2301 pad 2: OTG_ID -> GND
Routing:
- net GND: track 0.00 -> 484.2 mm, vias 0 -> 282
- net OTG_ID: track 437.5 -> 0.00 mm, vias 237 -> 0
- net +3V3_PWR_OUT: track 297.9 -> 0.00 mm, vias 18 -> 0
- net +1V8: track 411.5 -> 152.3 mm, vias 37 -> 64
- net +5V: track 245.3 -> 19.5 mm, vias 19 -> 0
- net +3V3: track 217.6 -> 113.4 mm, vias 42 -> 31
- net Net-(C14-Pad1): track 77.7 -> 0.00 mm
- net UART_TX_MIO15: track 67.2 -> 0.00 mm, vias 2 -> 0
- net /USB, SDIO, RJ45, JTAG, UART, I2C/USBA_P: track 64.8 -> 0.00 mm, vias 1 -> 0
- net /USB, SDIO, RJ45, JTAG, UART, I2C/USBA_N: track 64.8 -> 0.00 mm, vias 1 -> 0
- net UART_RX_MIO14: track 64.7 -> 0.00 mm, vias 2 -> 0
- net /lan9254/RUNLED: track 69.9 -> 16.6 mm, vias 4 -> 2
- net Net-(R2108-Pad2): track 2.14 -> 53.7 mm, vias 0 -> 2
- net Net-(R2107-Pad2): track 2.04 -> 50.1 mm, vias 0 -> 2
- net B13_L18_P: track 49.7 -> 1.94 mm, vias 2 -> 0
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- added copper zone on In2.Cu, net +1V0
- added copper zone on In2.Cu, net +1V8
- added copper zone on In2.Cu, net /fpga/1V0_MGT
- added copper zone on In2.Cu, net /fpga/1V2_MGT
- added copper zone on B.Cu, net GND
- added copper zone on In1.Cu, net GND
- removed copper zone on F.Cu, net +3V3
- removed copper zone on F.Cu, net +3V3_PWR_OUT
- removed copper zone on B.Cu, net +5V
- removed copper zone on F.Cu, net +5V
- removed copper zone on F.Cu, net Net-(L1101-Pad2)
- removed copper zone on B.Cu, net OTG_ID
- removed copper zone on F.Cu, net OTG_ID
- removed copper zone on In1.Cu, net OTG_ID
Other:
- net class Default: clearance 0.1524 -> 0.0889
- rule trace_clearance: 0.1524 -> 0.0889
